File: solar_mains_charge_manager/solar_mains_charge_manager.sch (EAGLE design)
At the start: 11 parts, among them T1 TIP122, X1 22-23-2031, X2 22-23-2021, X4 22-23-2031, X5 22-23-2031

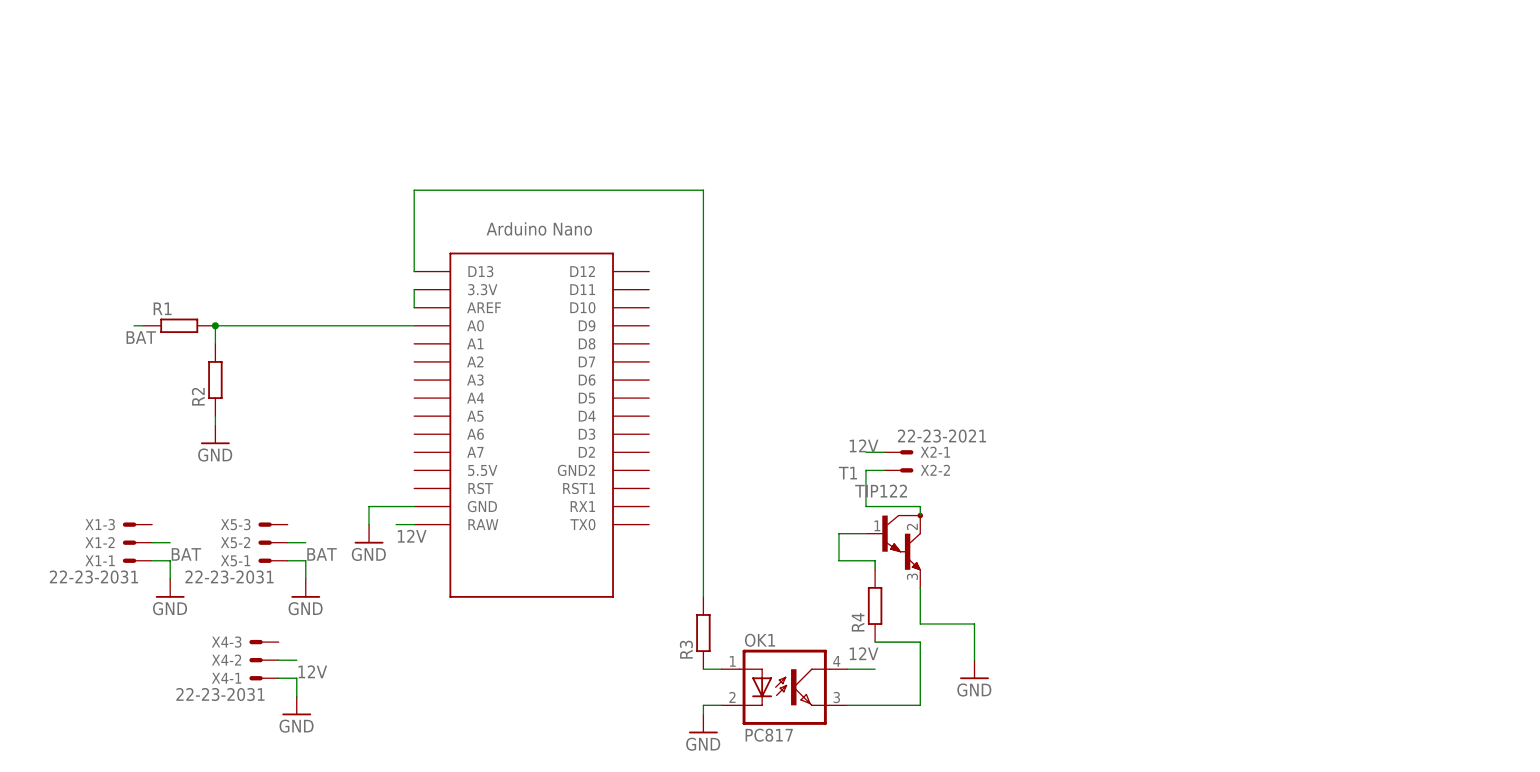
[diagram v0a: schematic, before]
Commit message: Some more schematic and spreadsheet
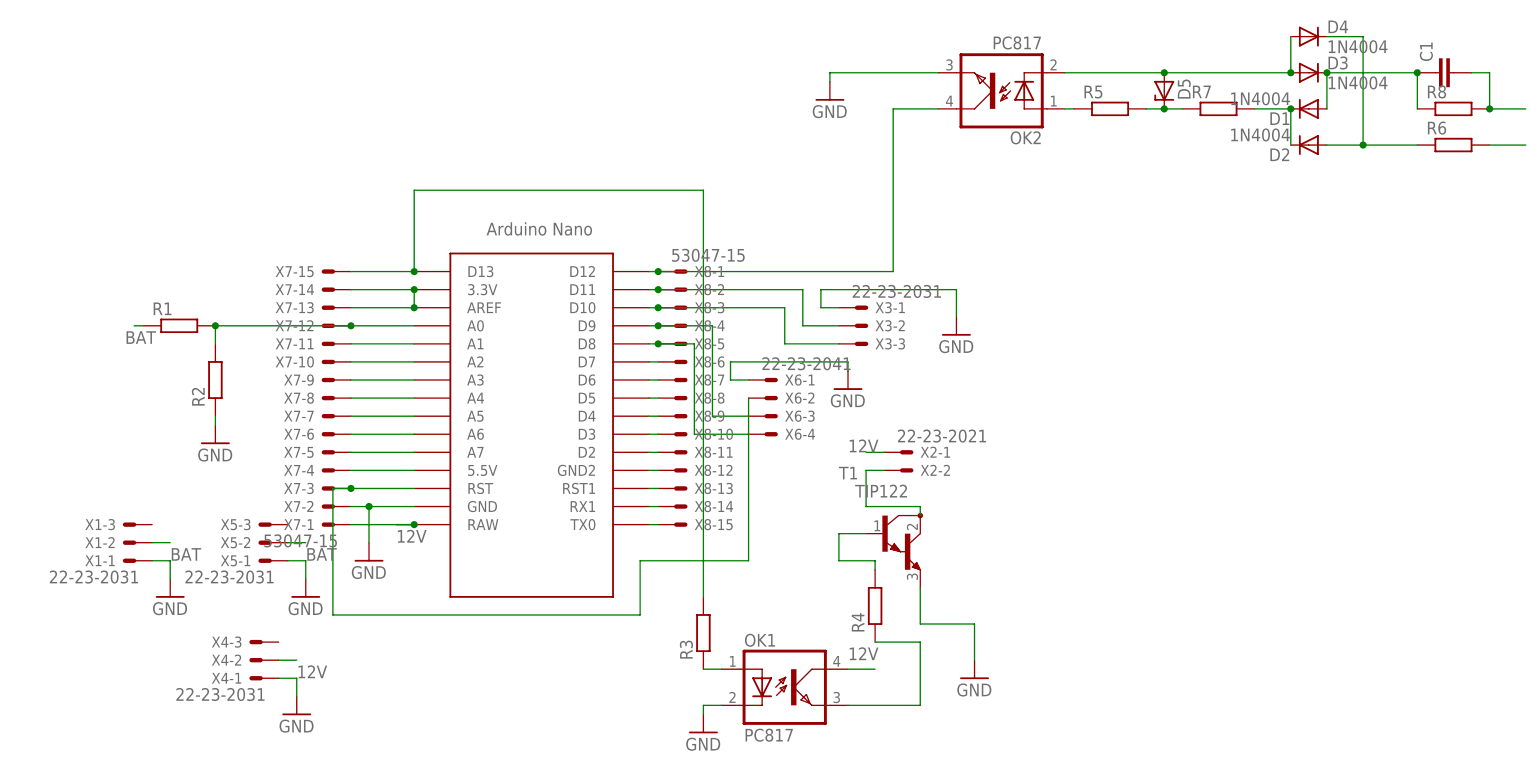
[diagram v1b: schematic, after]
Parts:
- added C1: (no value), capacitor-wima:C5/2.5
- added D1, D2, D3, D4: 1N4004, diode:1N4004
- added D5: (no value), diode:ZENER-DIODEDO34-7
- added OK2: PC817, optocoupler:PC817
- added R5: (no value), resistor:R-EU_0204/5
- added R6, R7, R8: (no value), resistor:R-EU_0204/7
- added X3: 22-23-2031, con-molex:22-23-2031
- added X6: 22-23-2041, con-molex:22-23-2041
- added X7, X8: 53047-15, con-molex:53047-15
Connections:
- new net N$10: D3.A, D4.A, D5.A, OK2.C
- new net N$11: D1.C, D2.C, R7.2
- new net N$12: OK2.COL, U$1.D12, X8-1.S
- new net N$13: C1.1, D1.A, D3.C, R8.1
- new net N$14: C1.2, R8.2
- new net N$15: D2.A, D4.C, R6.1
- new net N$16: R6.2
- new net N$17: U$1.D11, X3-2.S, X8-2.S
- new net N$18: U$1.D10, X3-3.S, X8-3.S
- new net N$19: U$1.D9, X6-3.S, X8-4.S
- new net N$20: U$1.D8, X6-4.S, X8-5.S
- new net N$21: U$1.RST, X6-2.S, X7-3.S
- new net N$22: U$1.D7, X8-6.S
- new net N$23: U$1.D6, X8-7.S
- new net N$24: U$1.D5, X8-8.S
- new net N$25: U$1.D4, X8-9.S
- new net N$26: U$1.D3, X8-10.S
- new net N$27: U$1.D2, X8-11.S
- new net N$28: U$1.GND2, X8-12.S
- new net N$29: U$1.RST1, X8-13.S
- new net N$30: U$1.RX1, X8-14.S
- new net N$31: U$1.TX0, X8-15.S
- new net N$32: U$1.5.5V, X7-4.S
- new net N$33: U$1.A7, X7-5.S
- new net N$34: U$1.A6, X7-6.S
- new net N$35: U$1.A5, X7-7.S
- new net N$36: U$1.A4, X7-8.S
- new net N$37: U$1.A3, X7-9.S
- new net N$38: U$1.A2, X7-10.S
- new net N$39: U$1.A1, X7-11.S
- new net N$8: OK2.A, R5.1
- new net N$9: D5.C, R5.2, R7.1
- net 12V: now also X7-1.S
- net GND: now also OK2.EMIT, X3-1.S, X6-1.S, X7-2.S
- net N$1: now also X7-13.S, X7-14.S
- net N$2: now also X7-15.S
- net N$3: now also X7-12.S
